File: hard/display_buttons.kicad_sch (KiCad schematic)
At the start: 12 parts, among them SW2 SW_MEC_5G, SW3 SW_MEC_5G, SW4 SW_MEC_5G, SW5 SW_MEC_5G

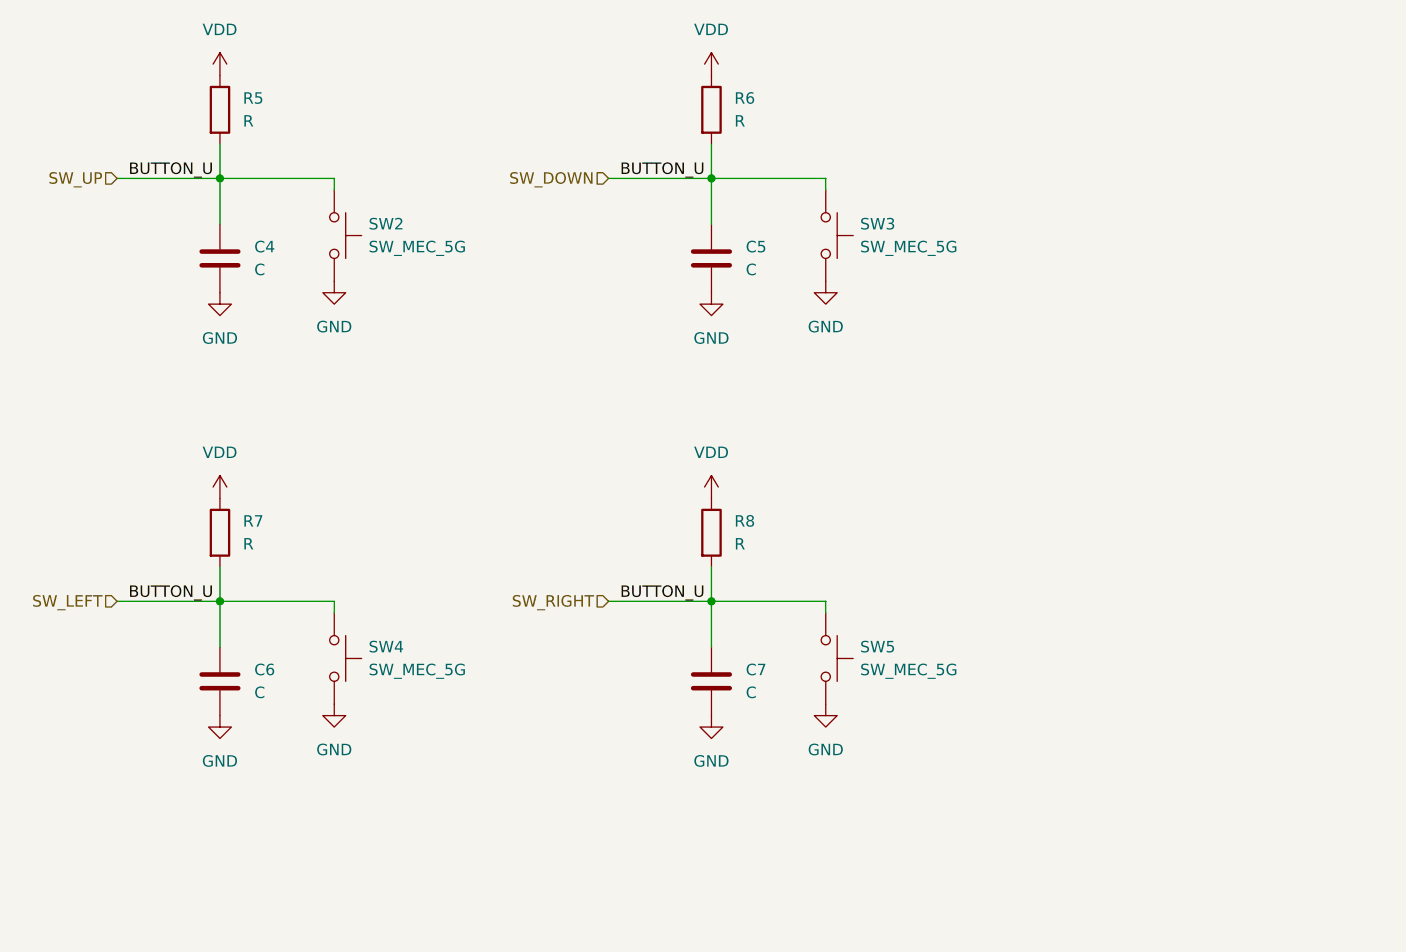
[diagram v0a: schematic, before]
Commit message: update
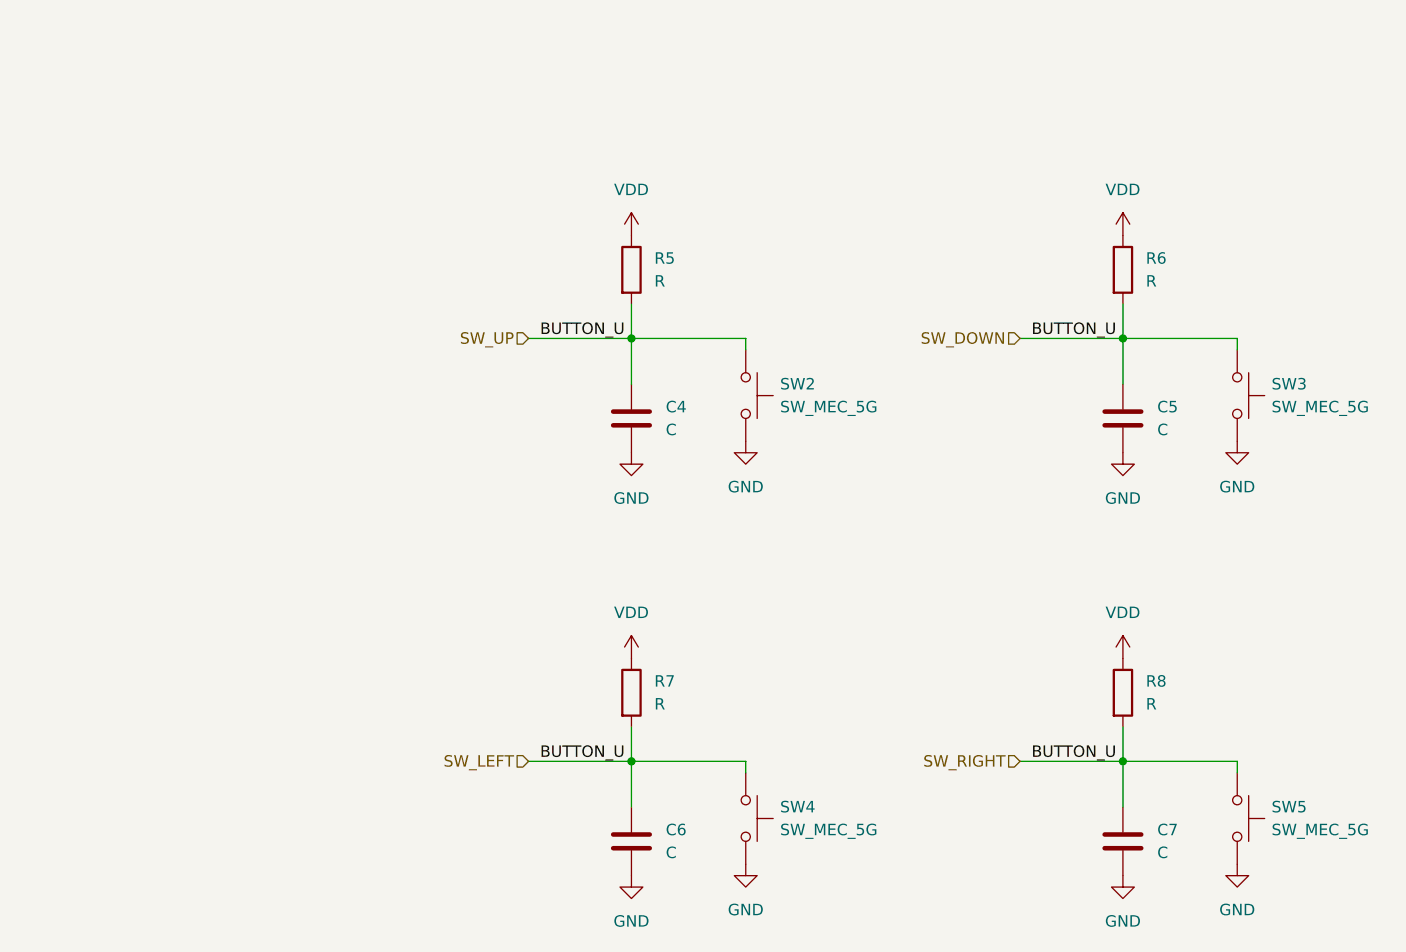
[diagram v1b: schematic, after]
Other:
- moved on the sheet: C4, C5, C6, C7, R5, R6, R7, R8, SW2, SW3, SW4, SW5
